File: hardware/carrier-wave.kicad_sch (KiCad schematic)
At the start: 4 parts, among them U2 OPA695, U3 THS3491, U4 AD9834, U7 TS5A3159ADCK

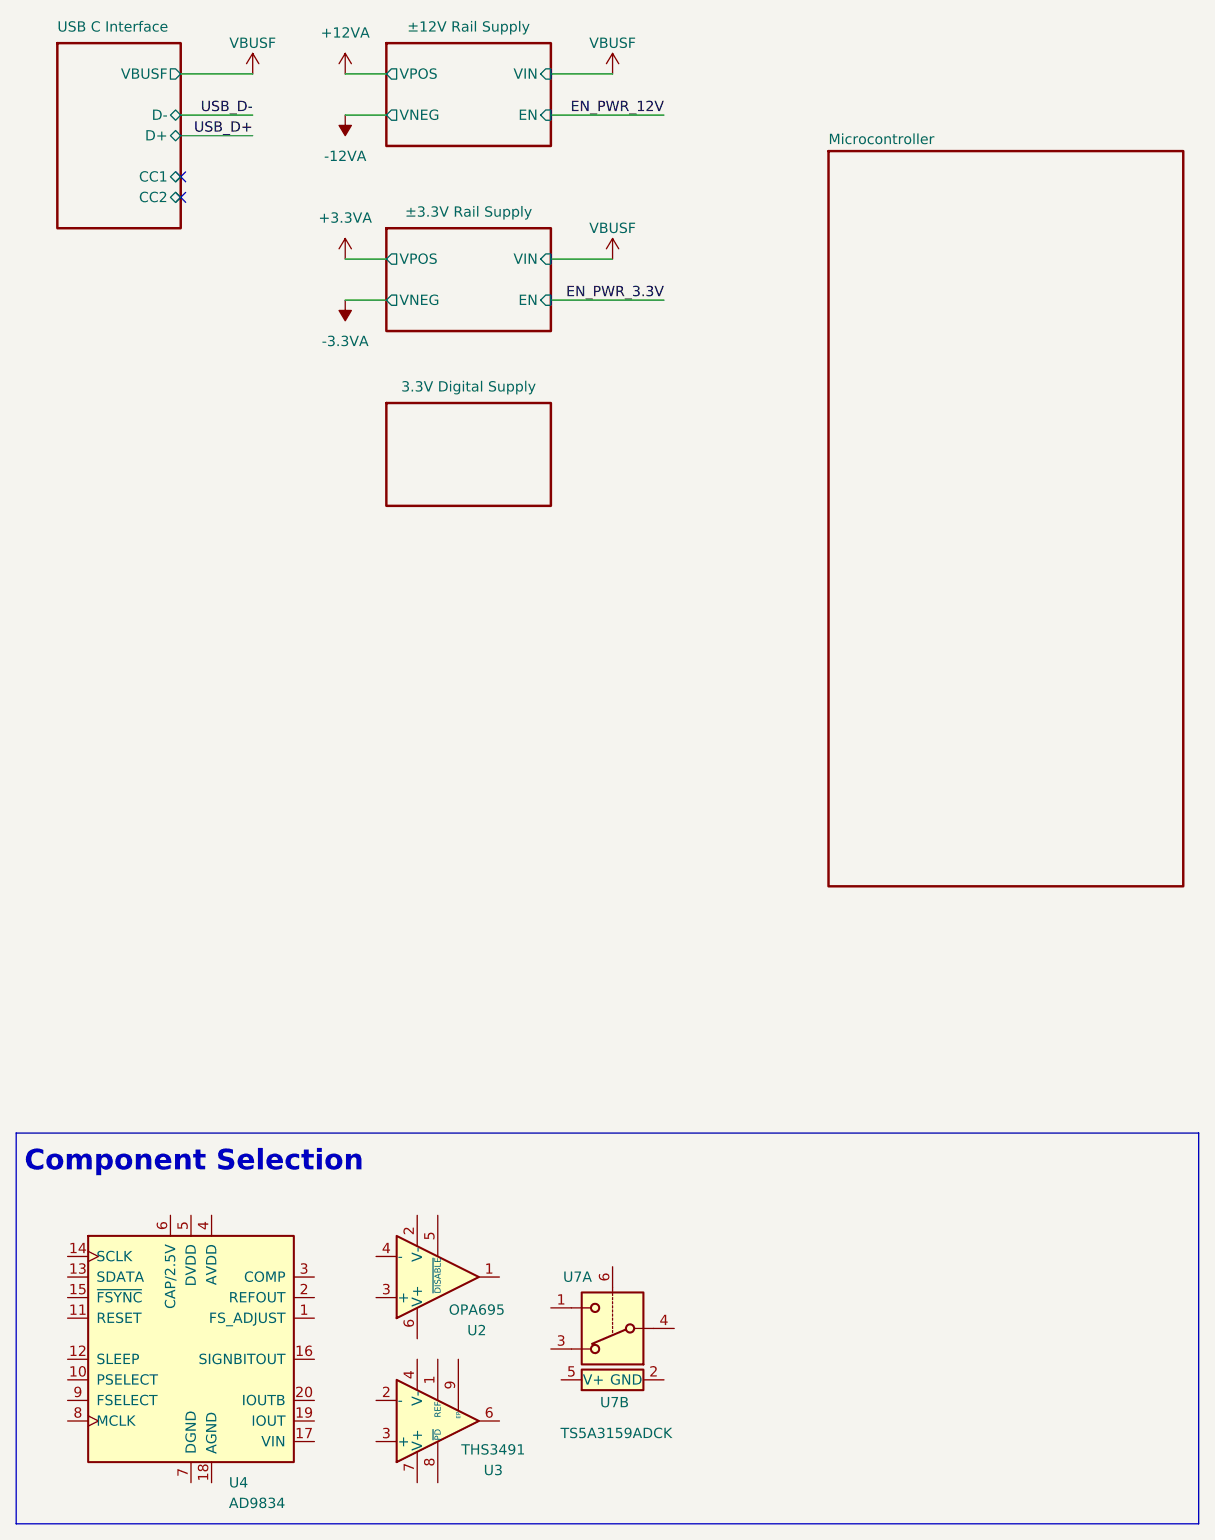
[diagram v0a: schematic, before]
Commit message: Finalize power
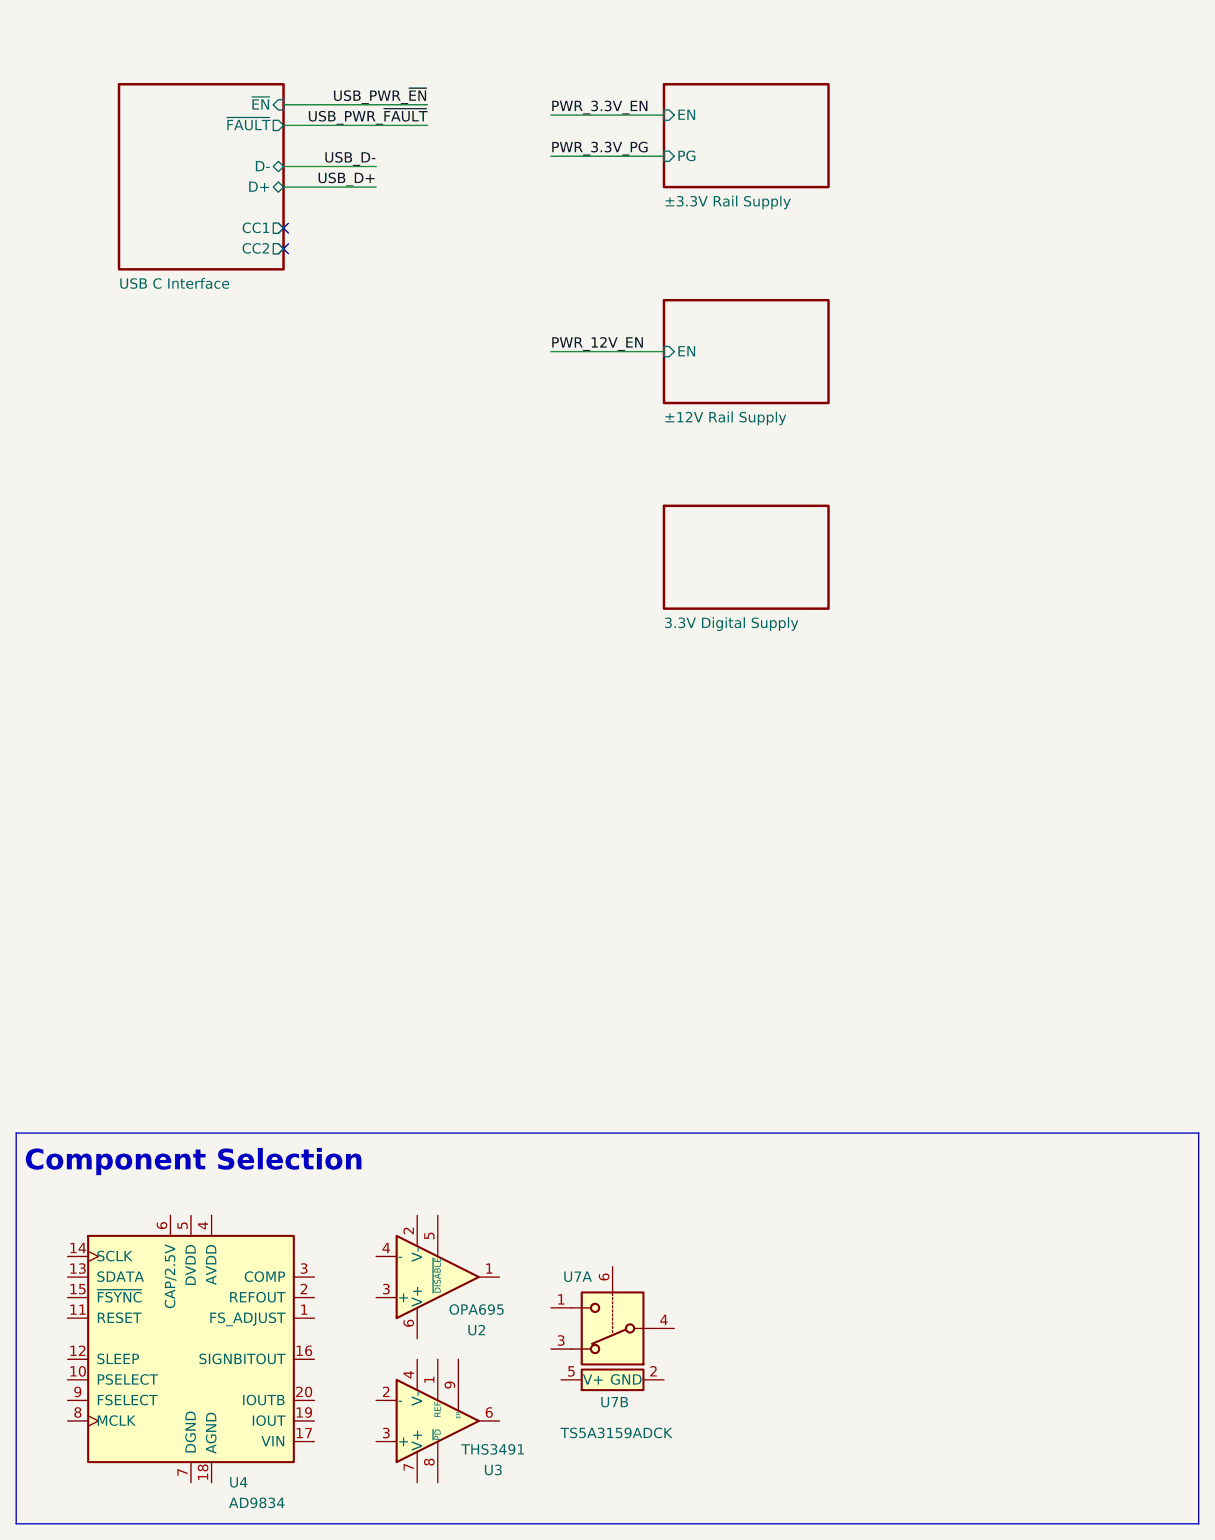
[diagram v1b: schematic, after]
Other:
- removed sheet Microcontroller
- sheet USB C Interface ports: added ~{EN}, ~{FAULT}; removed VBUSF
- sheet ±12V Rail Supply ports: added none; removed VIN, VNEG, VPOS
- sheet ±3.3V Rail Supply ports: added PG; removed VIN, VNEG, VPOS
